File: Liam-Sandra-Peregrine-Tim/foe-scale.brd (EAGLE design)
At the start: 100 x 80 mm, 40 parts, among them U1 LM311, U2 SAMD21E

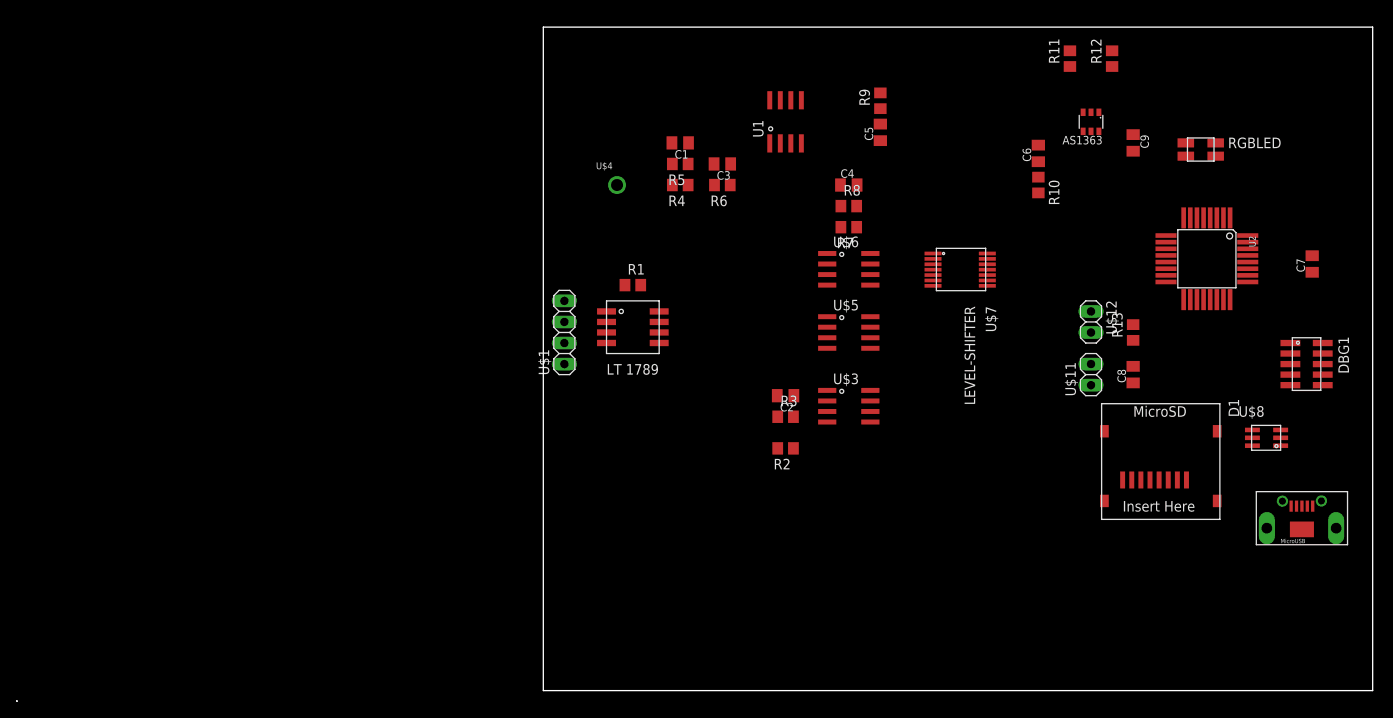
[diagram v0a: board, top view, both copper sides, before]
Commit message: minor changes
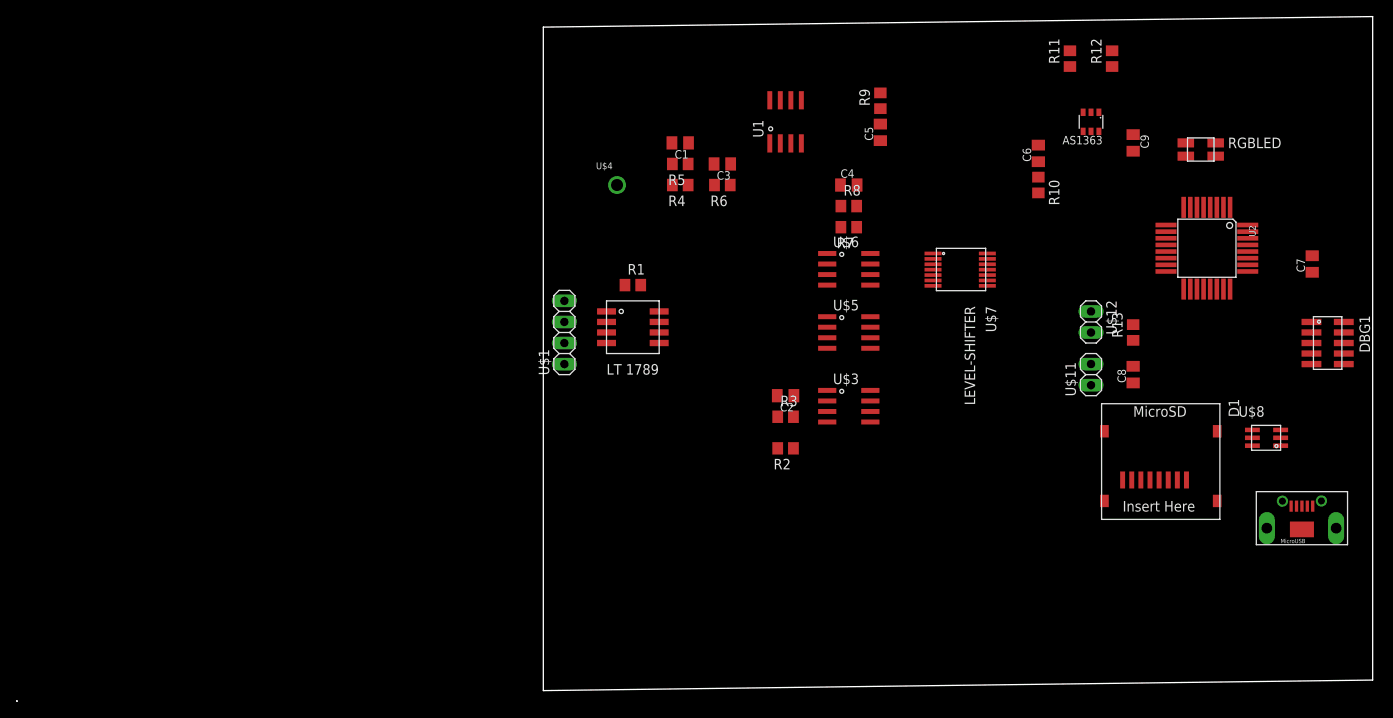
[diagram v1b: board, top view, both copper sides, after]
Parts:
- moved DBG1 3.59 mm to (96.5, 44.5)
- moved U2 1.27 mm to (80.0, 53.3)
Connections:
- removed net +3.3V: U$7.VCC
- removed net N$9: R10.2
- net 3.3V: now also R10.2, U$7.VCC
- net SCK-PA08: no longer U$7.IVCC1
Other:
- board size 100 x 80 mm -> 100 x 81.3 mm
